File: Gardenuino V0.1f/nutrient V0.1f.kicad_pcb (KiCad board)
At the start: 2 copper layers, 99.1 x 71.1 mm, 86 parts, among them J1 Conn_01x04_Male, J10 Conn_01x01_Male, J2 Conn_01x04_Female, J3 Conn_01x04_Male, J4 Conn_01x04_Male, J5 Conn_01x04_Female, J6 Conn_01x04_Male, J7 Conn_01x03_Male, J8 Conn_01x03_Male, J9 Conn_01x01_Male, P1 SolderJumper_2_Open, P2 SolderJumper_2_Bridged, P3 SolderJumper_2_Bridged, P4 SolderJumper_2_Bridged, Q1 Q_NMOS_DGS, Q10 Q_NMOS_DGS, Q2 Q_NMOS_DGS, Q3 Q_NMOS_DGS, Q4 Q_NMOS_DGS, Q5 Q_NMOS_DGS, Q6 Q_NMOS_DGS, Q7 Q_NMOS_DGS, Q8 2N3904, U1 23LC512, U2 DS1307+, Y1 Crystal_Small

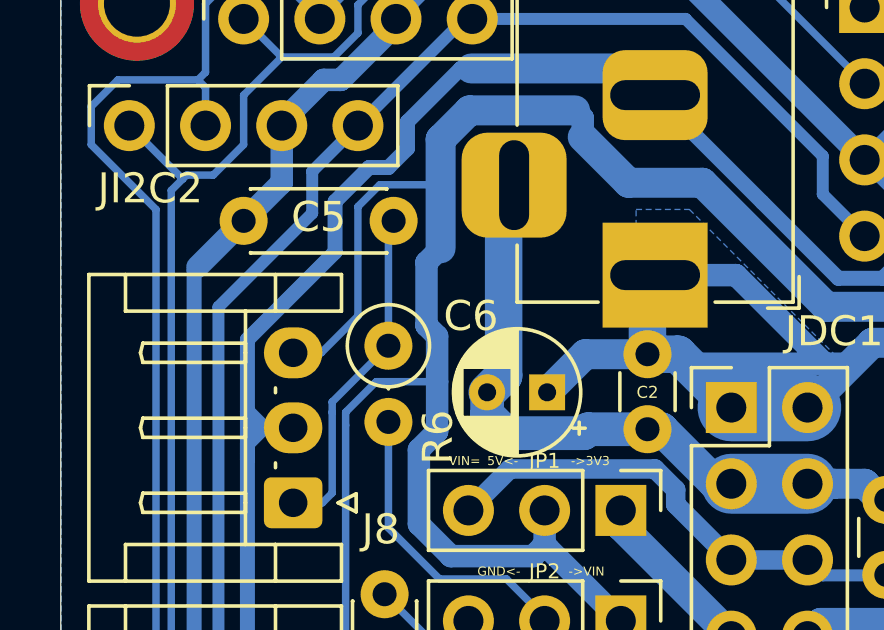
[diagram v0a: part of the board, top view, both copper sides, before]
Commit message: SpectDrone Development
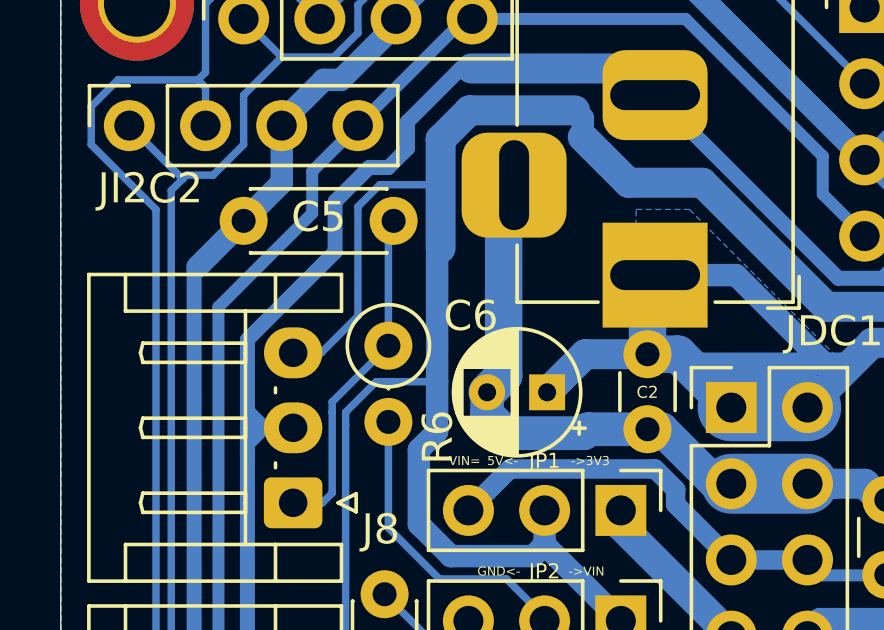
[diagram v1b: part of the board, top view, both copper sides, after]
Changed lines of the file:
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@@
   (segment locked (start 112.22999 41.85861) (end 113.1946 40.894) (width 1) (layer "B.Cu") (net 27))
   (segment locked (start 120.957482 43.307) (end 125.091471 47.440989) (width 1) (layer "B.Cu") (net 27))
-  (segment (start 112.22999 45.49149) (end 111.76 45.96148) (width 0.75) (layer "B.Cu") (net 27))
   (segment locked (start 107.315 60.024) (end 109.065021 58.273979) (width 0.25) (layer "B.Cu") (net 27))
   (segment (start 111.506 52.206853) (end 111.506 54.687002) (width 0.75) (layer "B.Cu") (net 27))
@@
   (segment locked (start 115.697 55.372) (end 115.57 55.499) (width 0.75) (layer "B.Cu") (net 27))
   (segment (start 116.967 41.783) (end 118.491 43.307) (width 1) (layer "B.Cu") (net 27))
-  (segment (start 111.76 45.96148) (end 111.76 48.065147) (width 0.75) (layer "B.Cu") (net 27))
   (segment locked (start 189.54501 38.82399) (end 189.54501 73.34499) (width 1) (layer "B.Cu") (net 27))
   (segment locked (start 115.57 55.499) (end 115.316 55.753) (width 0.75) (layer "B.Cu") (net 27))
-  (segment (start 112.113489 48.418636) (end 112.113489 49.938511) (width 0.75) (layer "B.Cu") (net 27))
   (segment locked (start 118.237 60.2615) (end 118.237 61.595) (width 0.75) (layer "B.Cu") (net 27))
   (segment (start 116.967 41.148) (end 116.713 40.894) (width 0.75) (layer "B.Cu") (net 27))
@@
   (segment (start 112.113489 51.599364) (end 111.506 52.206853) (width 0.75) (layer "B.Cu") (net 27))
   (segment locked (start 115.57 55.499) (end 115.824 55.499) (width 0.75) (layer "B.Cu") (net 27))
+  (segment (start 112.22999 45.49149) (end 112.113489 45.607991) (width 0.75) (layer "B.Cu") (net 27))
   (segment locked (start 127.539611 47.440989) (end 137.322611 37.657989) (width 1) (layer "B.Cu") (net 27))
   (segment locked (start 115.316 55.753) (end 112.571998 55.753) (width 0.75) (layer "B.Cu") (net 27))
@@
   (segment locked (start 124.46 60.96) (end 123.2 59.7) (width 0.4) (layer "B.Cu") (net 27))
   (segment locked (start 189.611 76.327) (end 189.611 95.227) (width 1) (layer "B.Cu") (net 27))
-  (segment (start 111.76 48.065147) (end 112.113489 48.418636) (width 0.75) (layer "B.Cu") (net 27))
   (segment (start 109.065021 50.954979) (end 110.081489 49.938511) (width 0.25) (layer "B.Cu") (net 27))
   (segment locked (start 112.571998 55.753) (end 111.506 54.687002) (width 0.75) (layer "B.Cu") (net 27))
+  (segment (start 112.113489 45.607991) (end 112.113489 49.938511) (width 0.75) (layer "B.Cu") (net 27))
   (segment locked (start 118.237 59.69) (end 118.7985 59.69) (width 0.75) (layer "B.Cu") (net 27))
   (segment locked (start 189.611 95.227) (end 185.672 95.227) (width 1) (layer "B.Cu") (net 27))
